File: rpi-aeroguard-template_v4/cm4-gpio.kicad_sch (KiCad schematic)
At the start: 29 parts, among them J2 Conn_01x02_Pin, J3 Conn_01x04_Pin, J4 Conn_01x02_Pin, J6 Conn_01x05_Pin, U1 TPS63070RNMR, U2 74LVC1G07SE-7

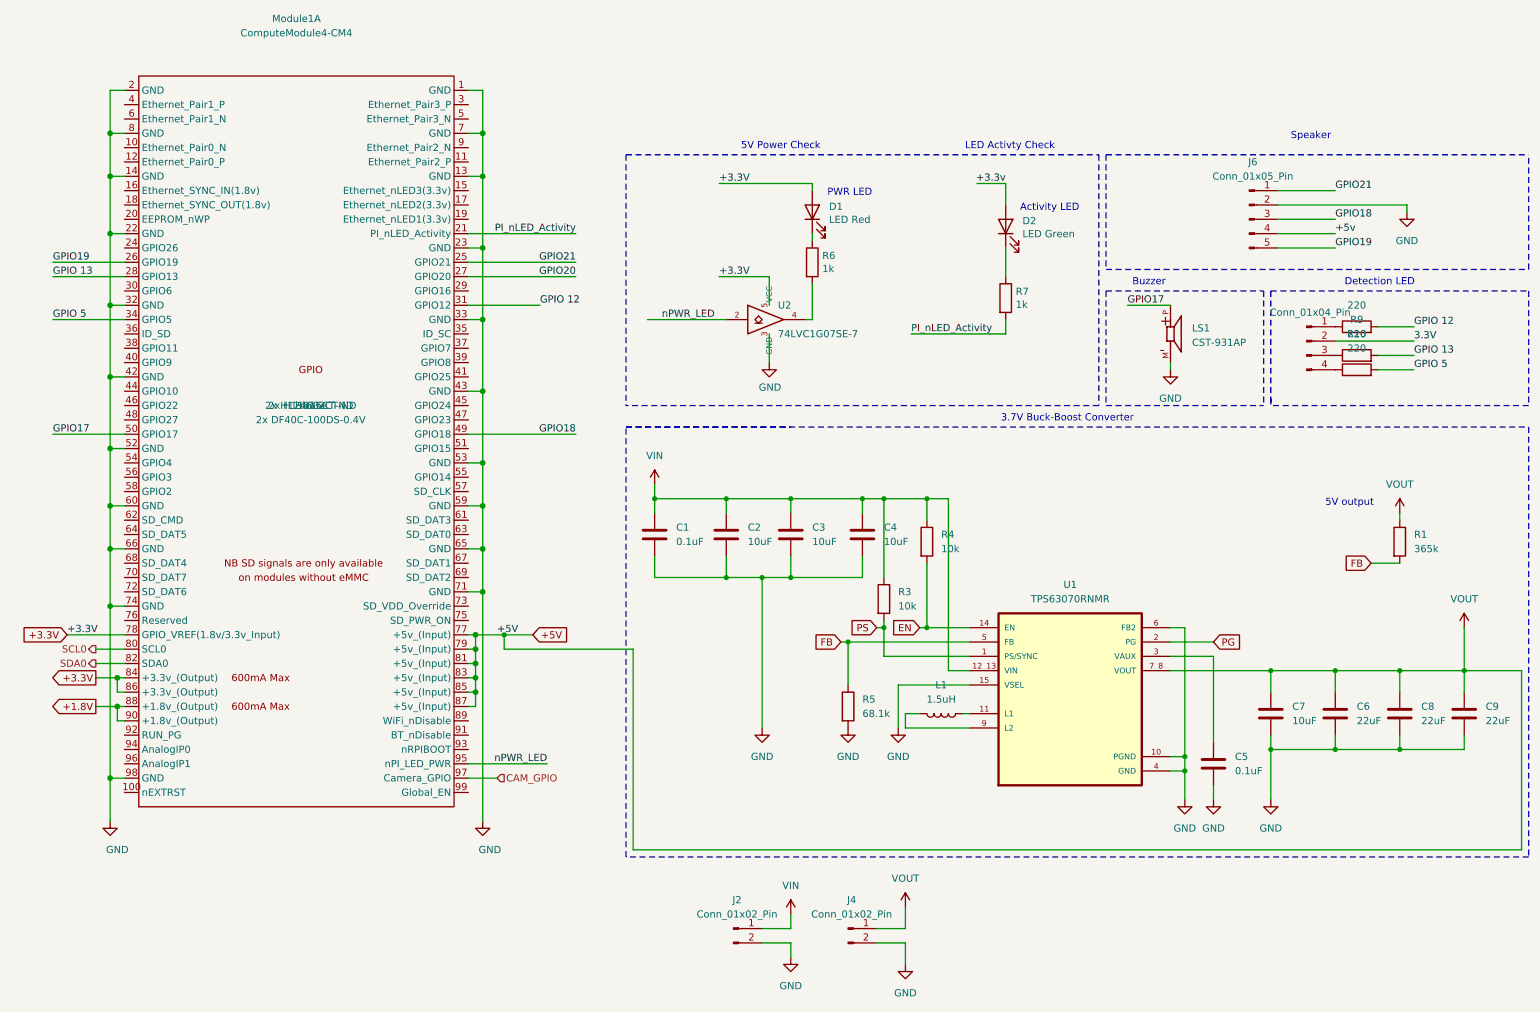
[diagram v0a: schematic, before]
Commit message: Add files via upload
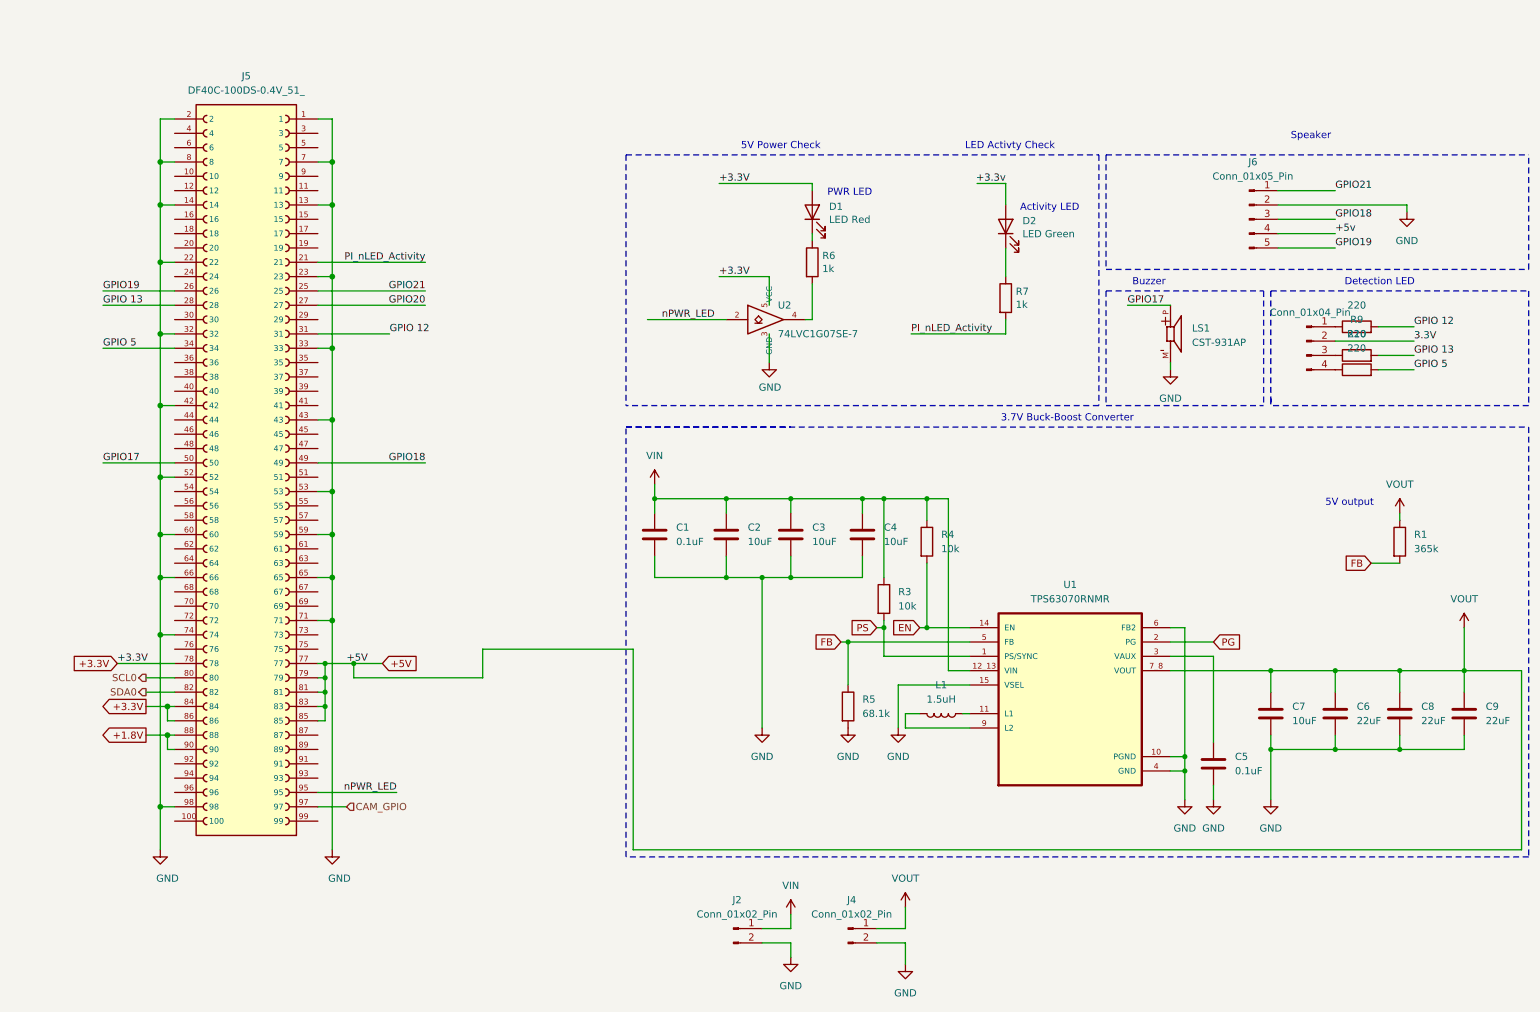
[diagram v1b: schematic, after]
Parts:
- removed Module1: ComputeModule4-CM4, CM4IO:Raspberry-Pi-4-Compute-Module, symbol CM4IO:ComputeModule4-CM4
- added J5: DF40C-100DS-0.4V_51_, DF40C-100DS-0.4V_51_:HIROSE_DF40C-100DS-0.4V_51_, symbol DF40C-100DS-0.4V_51_:DF40C-100DS-0.4V_51_
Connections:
- net +1.8V: now also J5.88, J5.90
- net +3.3V: now also J5.78, J5.84, J5.86
- net CAM_GPIO: now also J5.97
- net GND: now also J5.1, J5.13, J5.14, J5.2, J5.22, J5.23, J5.32, J5.33, J5.42, J5.43, J5.52, J5.53, J5.59, J5.60, J5.65, J5.66, J5.7, J5.71, J5.74, J5.8, J5.98
- net GPIO 12: now also J5.31
- net GPIO 13: now also J5.28
- net GPIO 5: now also J5.34
- net GPIO17: now also J5.50
- net GPIO18: now also J5.49
- net GPIO19: now also J5.26
- net GPIO20: now also J5.27
- net GPIO21: now also J5.25
- net PI_nLED_Activity: now also J5.21
- net SCL0: now also J5.80
- net SDA0: now also J5.82
- net VOUT: now also J5.77, J5.79, J5.81, J5.83, J5.85
- net nPWR_LED: now also J5.95
